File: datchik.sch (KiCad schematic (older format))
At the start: 1 part

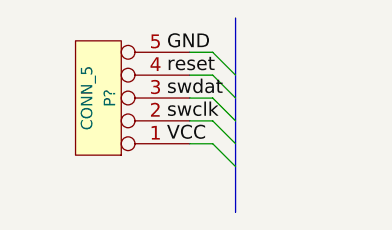
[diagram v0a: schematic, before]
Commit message: добавлена печатная плата
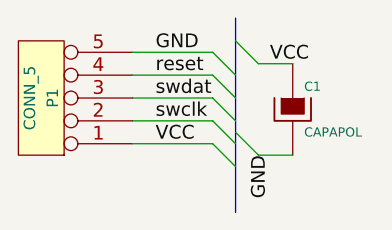
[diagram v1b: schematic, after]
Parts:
- added C1: CAPAPOL, ~, symbol CAPAPOL
- gave numbers to parts that had none: 1
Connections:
- net GND: now also P1.5, C1.2
- net VCC: now also P1.1, C1.1
- net reset: now also P1.4
- net swclk: now also P1.2
- net swdat: now also P1.3
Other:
- moved on the sheet: P1
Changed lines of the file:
@@
 $EndDescr
 $Comp
-L CONN_5 P?
+L CONN_5 P1
 U 1 1 545221CE
-P 900 1100
-F 0 "P?" V 850 1100 50  0000 C CNN
-F 1 "CONN_5" V 950 1100 50  0000 C CNN
-F 2 "" H 900 1100 60  0000 C CNN
-F 3 "" H 900 1100 60  0000 C CNN
-	1    900  1100
+P 650 1100
+F 0 "P1" V 600 1100 50  0000 C CNN
+F 1 "CONN_5" V 700 1100 50  0000 C CNN
+F 2 "" H 650 1100 60  0000 C CNN
+F 3 "" H 650 1100 60  0000 C CNN
+	1    650  1100
 	-1   0    0    1
 $EndComp
@@
 	1400 1000 1500 1100
 Wire Wire Line
-	1300 900  1400 900
+	1050 900  1400 900
 Wire Wire Line
-	1300 1000 1400 1000
+	1050 1000 1400 1000
 Wire Wire Line
-	1300 1100 1400 1100
+	1050 1100 1400 1100
 Wire Wire Line
-	1300 1200 1400 1200
+	1050 1200 1400 1200
 Wire Wire Line
-	1300 1300 1400 1300
-Text Label 1200 1300 0    60   ~ 0
+	1050 1300 1400 1300
+Text Label 1150 1300 0    60   ~ 0
 VCC
-Text Label 1200 1200 0    60   ~ 0
+Text Label 1150 1200 0    60   ~ 0
 swclk
-Text Label 1200 1100 0    60   ~ 0
+Text Label 1150 1100 0    60   ~ 0
 swdat
-Text Label 1200 1000 0    60   ~ 0
+Text Label 1150 1000 0    60   ~ 0
 reset
-Text Label 1200 900  0    60   ~ 0
+Text Label 1150 900  0    60   ~ 0
+GND
+$Comp
+L CAPAPOL C1
+U 1 1 54522450
+P 1750 1150
+F 0 "C1" H 1800 1250 40  0000 L CNN
+F 1 "CAPAPOL" H 1800 1050 40  0000 L CNN
+F 2 "~" H 1850 1000 30  0000 C CNN
+F 3 "~" H 1750 1150 300 0000 C CNN
+	1    1750 1150
+	1    0    0    -1
+$EndComp
+Entry Wire Line
+	1500 1250 1600 1350
+Entry Wire Line
+	1500 850  1600 950
+Wire Wire Line
+	1600 950  1750 950
+Wire Wire Line
+	1600 1350 1750 1350
+Text Label 1650 950  0    60   ~ 0
+VCC
+Text Label 1650 1350 3    60   ~ 0
 GND
 $EndSCHEMATC
